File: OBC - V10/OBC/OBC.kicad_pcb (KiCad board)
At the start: 4 copper layers, 42 x 42 mm, 73 parts, among them J1 Conn_01x05, J2 Conn_01x04, J3 ESL_PQ_MainHeader, J4 Conn_02x20_Odd_Even, J6 Micro_SD_Card, U1 STM32L496VGTxP, U3 LSM9DS1TR, U4 LTC2850HDD#PBF, Y3 32.768 kHz, Y4 80 MHz

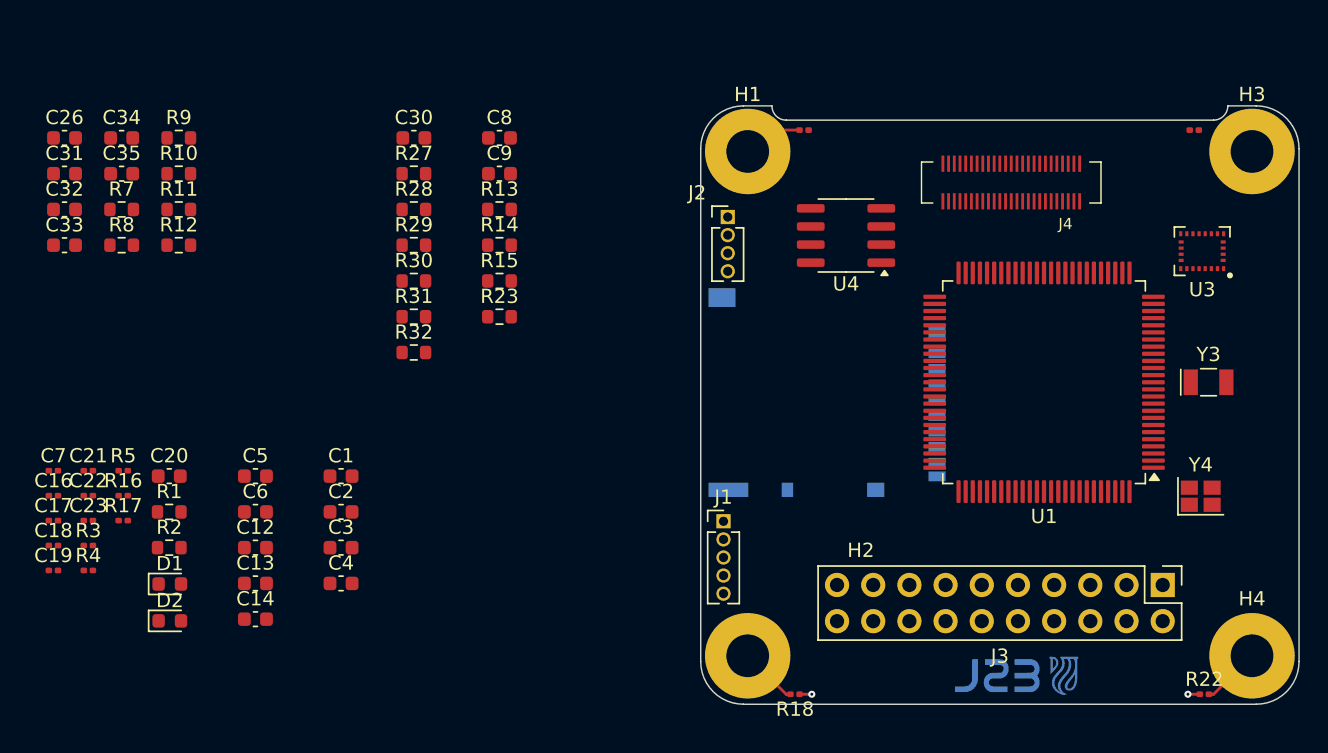
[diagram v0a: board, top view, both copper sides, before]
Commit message: PQ V12
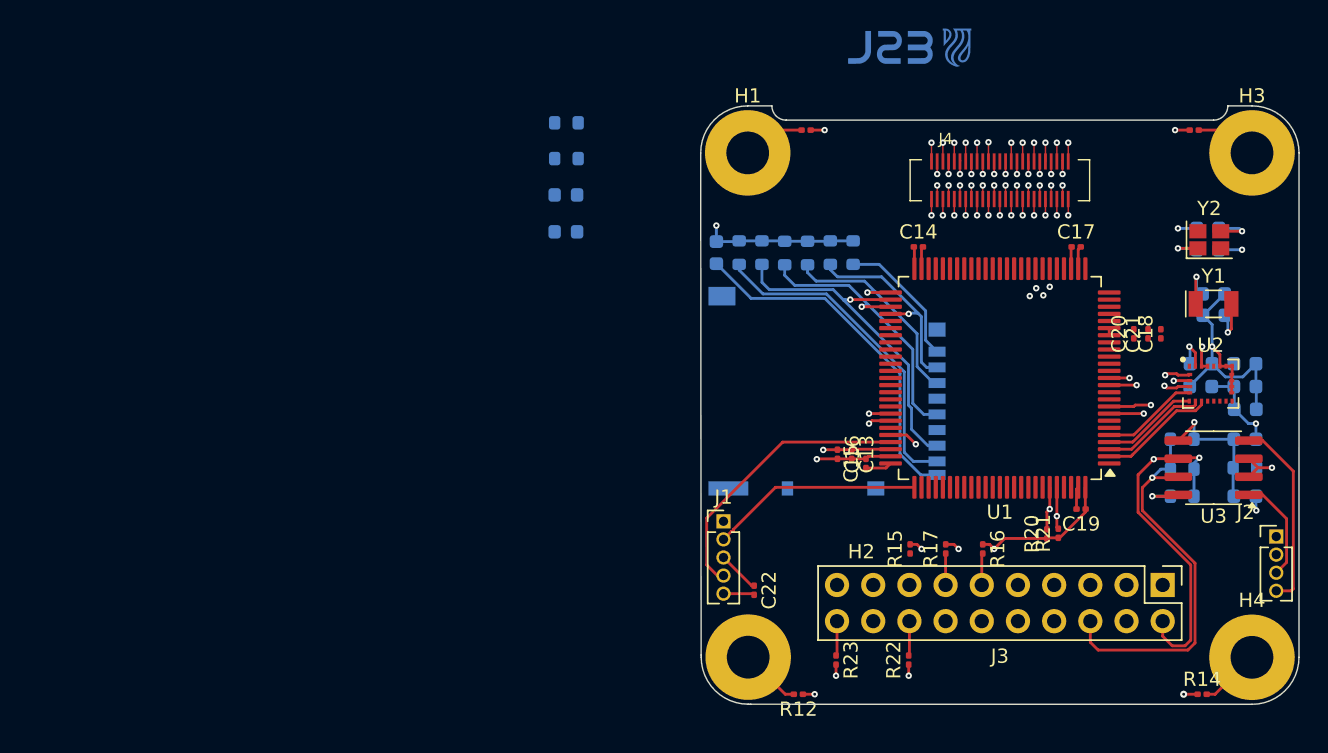
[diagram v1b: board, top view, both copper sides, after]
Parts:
- removed C26, C31, C32, C33, C34, C35: 220p, Capacitor_SMD:C_0603_1608Metric
- removed the R10 at (191.9, 27.6)
- removed the R11 at (191.9, 30.1)
- removed the R12 at (191.9, 32.6)
- removed the R7 at (187.9, 30.1)
- removed the R8 at (187.9, 32.6)
- removed the R9 at (191.9, 25.1)
- added C21: 1u, Skripsie:C_0201_0603Metric, F.Cu at (259.9, 38.8)
- added R22: 4k7, Skripsie:R_0201_0603Metric, F.Cu at (243.1, 61.7)
- added R23: 4k7, Skripsie:R_0201_0603Metric, F.Cu at (238.0, 61.7)
- C1: renamed from C30; moved to B.Cu
- C10: renamed from C6; moved to B.Cu
- C11: renamed from C8; moved to B.Cu
- C12: renamed from C9; moved to B.Cu
- C17: renamed from C20; footprint Capacitor_SMD:C_0603_1608Metric -> Skripsie:C_0201_0603Metric
- C2: renamed from C1; moved to B.Cu
- C20: renamed from C23; value 100n -> 1u
- C3: renamed from C2; moved to B.Cu
- C4: renamed from C3; moved to B.Cu
- C5: renamed from C4; moved to B.Cu
- C6: renamed from C12; moved to B.Cu
- C7: renamed from C13; moved to B.Cu
- C8: renamed from C14; moved to B.Cu
- C9: renamed from C5; moved to B.Cu
- D1, D2: moved to B.Cu
- R1: renamed from R27; moved to B.Cu
- R10: renamed from R23; moved to B.Cu
- R18: renamed from R1; moved to B.Cu
- R19: renamed from R2; moved to B.Cu
- R2: renamed from R28; moved to B.Cu
- R20: renamed from R16; value R -> 4k7
- R21: renamed from R17; value R -> 4k7
- R3: renamed from R29; moved to B.Cu
- R4: renamed from R30; moved to B.Cu
- R5: renamed from R31; moved to B.Cu
- R6: renamed from R32; moved to B.Cu
- R7: renamed from R13; moved to B.Cu
- R8: renamed from R14; moved to B.Cu
- R9: renamed from R15; moved to B.Cu
- U1: value STM32L496VGTxP -> STM32L496VGTx
- U3: renamed from U4; value LTC2850HDD#PBF -> MAX485EDA
- Y2: renamed from Y4; value 80 MHz -> 16 MHz
- moved C18 75.9 mm to (260.8, 38.8), turned to 90 degrees
- moved C20 74.5 mm to (258.9, 38.8), turned to 90 degrees
- moved C8 71.0 mm to (266.7, 44.1)
- moved C6 70.4 mm to (266.7, 42.5), turned to 180 degrees
- moved C9 69.9 mm to (266.7, 40.9), turned to 180 degrees
- moved C19 69.7 mm to (255.2, 51.1), turned to 180 degrees
- moved C7 67.8 mm to (263.6, 42.5), turned to 180 degrees
- moved C10 67.2 mm to (263.6, 40.9)
- moved C5 65.8 mm to (264.1, 31.4)
- moved C17 65.7 mm to (254.9, 32.7)
- moved R21 65.6 mm to (253.6, 52.8), turned to 90 degrees
- moved R20 64.9 mm to (252.8, 52.8), turned to 90 degrees
- moved C4 64.3 mm to (264.1, 32.9), turned to 180 degrees
- moved C14 63.7 mm to (243.8, 32.7)
- moved C3 62.8 mm to (264.5, 37.5)
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- renumbered C16 to C13, C17 to C14, C18 to C15, C19 to C16, C21 to C18, C22 to C19, C7 to C22, J6 to J5, R6 to R11, R18 to R12, R21 to R13, R22 to R14, R3 to R15, R4 to R16, R5 to R17, U3 to U2, Y3 to Y1
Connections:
- net EPS_RST renamed EPS-RST
- C22 pad 1: NRST -> GND
- C22 pad 2: GND -> NRST
- U1 pad 15: unconnected-(U1-PC0-Pad15) -> I2C-SCL
- U1 pad 16: unconnected-(U1-PC1-Pad16) -> I2C-SDA
- U1 pad 17: PWR -> DB
- U1 pad 18: TX -> DB
- U1 pad 2: unconnected-(U1-PE3-Pad2) -> CSM
- U1 pad 20: unconnected-(U1-VREF--Pad20) -> GND
- U1 pad 21: unconnected-(U1-VREF+-Pad21) -> DCap
- U1 pad 23: OPA1 -> DB
- U1 pad 24: OPA2 -> DB
- U1 pad 25: OPA3 -> DB
- U1 pad 26: OPA4 -> DB
- U1 pad 29: OPA6 -> unconnected-(U1-PA4-Pad29)
- U1 pad 3: unconnected-(U1-PE4-Pad3) -> CSAG
- U1 pad 30: OPA5 -> unconnected-(U1-PA5-Pad30)
- U1 pad 31: unconnected-(U1-PA6-Pad31) -> DB
- U1 pad 32: unconnected-(U1-PA7-Pad32) -> DB
- U1 pad 33: USART TX -> DB
- U1 pad 34: USART RX -> DB
- U1 pad 35: RS-EN -> DB
- U1 pad 36: unconnected-(U1-PB1-Pad36) -> DB
- U1 pad 4: unconnected-(U1-PE5-Pad4) -> SAOM
- U1 pad 43: SPI NSS -> DB
- U1 pad 44: SPI SCK -> DB
- U1 pad 45: SPI MISO -> DB
- U1 pad 46: SPI MOSI -> DB
- U1 pad 47: unconnected-(U1-PB10-Pad47) -> DB
- U1 pad 48: DCap -> DB
- U1 pad 5: unconnected-(U1-PE6-Pad5) -> SAOG
- U1 pad 51: PPS -> SPI MOSI
- U1 pad 52: I2C-SCL -> SPI MISO
- U1 pad 53: I2C-SDA -> SPI SCK
- U1 pad 54: unconnected-(U1-PB15-Pad54) -> SPI NSS
- U1 pad 55: unconnected-(U1-PD8-Pad55) -> DB
- U1 pad 56: unconnected-(U1-PD9-Pad56) -> DB
- U1 pad 59: unconnected-(U1-PD12-Pad59) -> I2C-SDA
- U1 pad 60: unconnected-(U1-PD13-Pad60) -> I2C-SCL
- U1 pad 71: unconnected-(U1-PA12-Pad71) -> RS-EN
- U1 pad 77: unconnected-(U1-PA15-Pad77) -> DB
- U1 pad 78: unconnected-(U1-PC10-Pad78) -> DB
- U1 pad 79: unconnected-(U1-PC11-Pad79) -> DB
- U1 pad 80: unconnected-(U1-PC12-Pad80) -> DB
- U1 pad 81: unconnected-(U1-PD0-Pad81) -> DB
- U1 pad 82: unconnected-(U1-PD1-Pad82) -> DB
- U1 pad 83: unconnected-(U1-PD2-Pad83) -> DB
- U1 pad 86: unconnected-(U1-PD5-Pad86) -> DB
- U1 pad 87: unconnected-(U1-PD6-Pad87) -> DB
- U1 pad 89: unconnected-(U1-PB3-Pad89) -> DB
- U1 pad 90: unconnected-(U1-PB4-Pad90) -> DB
- U1 pad 91: SCL -> DB
- U1 pad 92: SDA -> unconnected-(U1-PB6-Pad92)
- U1 pad 93: CSM -> unconnected-(U1-PB7-Pad93)
- U1 pad 94: CSAG -> unconnected-(U1-PH3-Pad94)
- U1 pad 95: SAOM -> SCL
- U1 pad 96: SAOG -> SDA
- U1 pad 98: DCap -> unconnected-(U1-PE1-Pad98)
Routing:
- net GND: track 1.70 -> 74.4 mm, vias 2 -> 9
- net USART RX: track 0.00 -> 50.9 mm, vias 0 -> 1
- net DCap: track 0.00 -> 47.5 mm, vias 0 -> 12
- net USART TX: track 0.00 -> 44.8 mm, vias 0 -> 1
- net RS-EN: track 0.00 -> 41.5 mm, vias 0 -> 2
- net RS-B: track 0.00 -> 28.2 mm, vias 0 -> 1
- net RS-A: track 0.00 -> 24.4 mm, vias 0 -> 2
- net SPI MISO: track 0.00 -> 24.2 mm, vias 0 -> 1
- net Net-(J5-DAT1): track 0.00 -> 23.2 mm
- net /Daughterboard Connector/DB8: track 0.00 -> 22.8 mm, vias 0 -> 3
- net OSC_OUT: track 0.00 -> 21.0 mm, vias 0 -> 2
- net SPI SCK: track 0.00 -> 20.3 mm, vias 0 -> 1
- net SWDIO: track 0.00 -> 19.9 mm
- net /Daughterboard Connector/DB4: track 0.00 -> 19.6 mm, vias 0 -> 3
- net SCL: track 0.00 -> 19.3 mm, vias 0 -> 2
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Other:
- outline, holes or cut-outs redrawn
